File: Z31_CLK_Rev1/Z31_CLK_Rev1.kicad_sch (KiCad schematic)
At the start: 16 parts, among them J1 Conn_01x06_Male, J2 ICSP, U1 MAX6922, U2 4BT-78Z_6L, U3 ATMEGA328-AURCT-ND, U4 MCP2510, U5 TJR1443, Y1 8MHz, Y2 16MHz

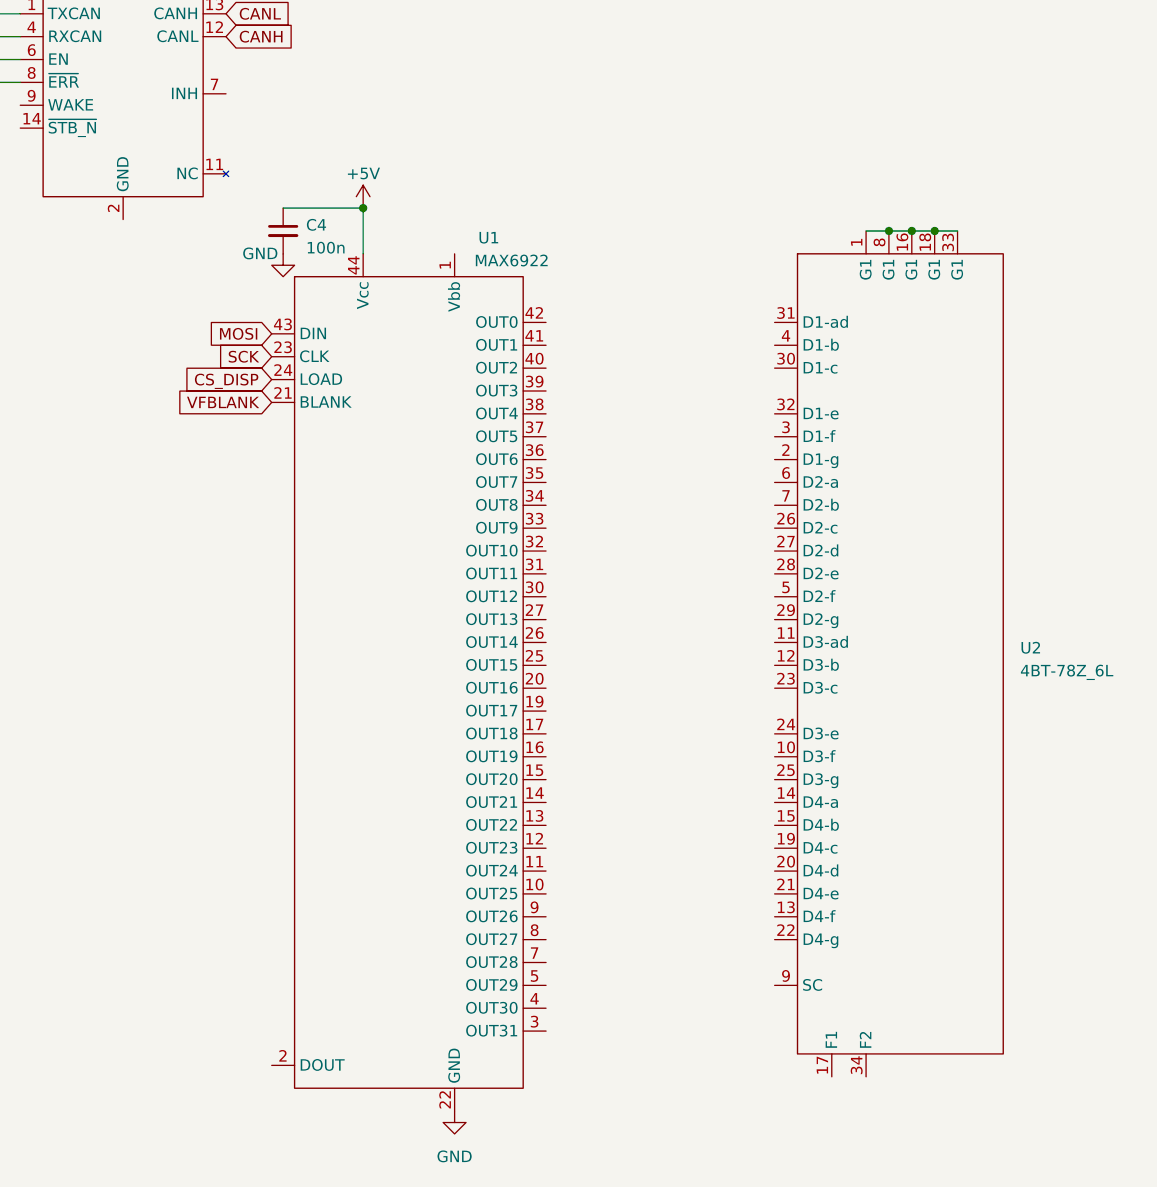
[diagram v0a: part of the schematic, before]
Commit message: add code
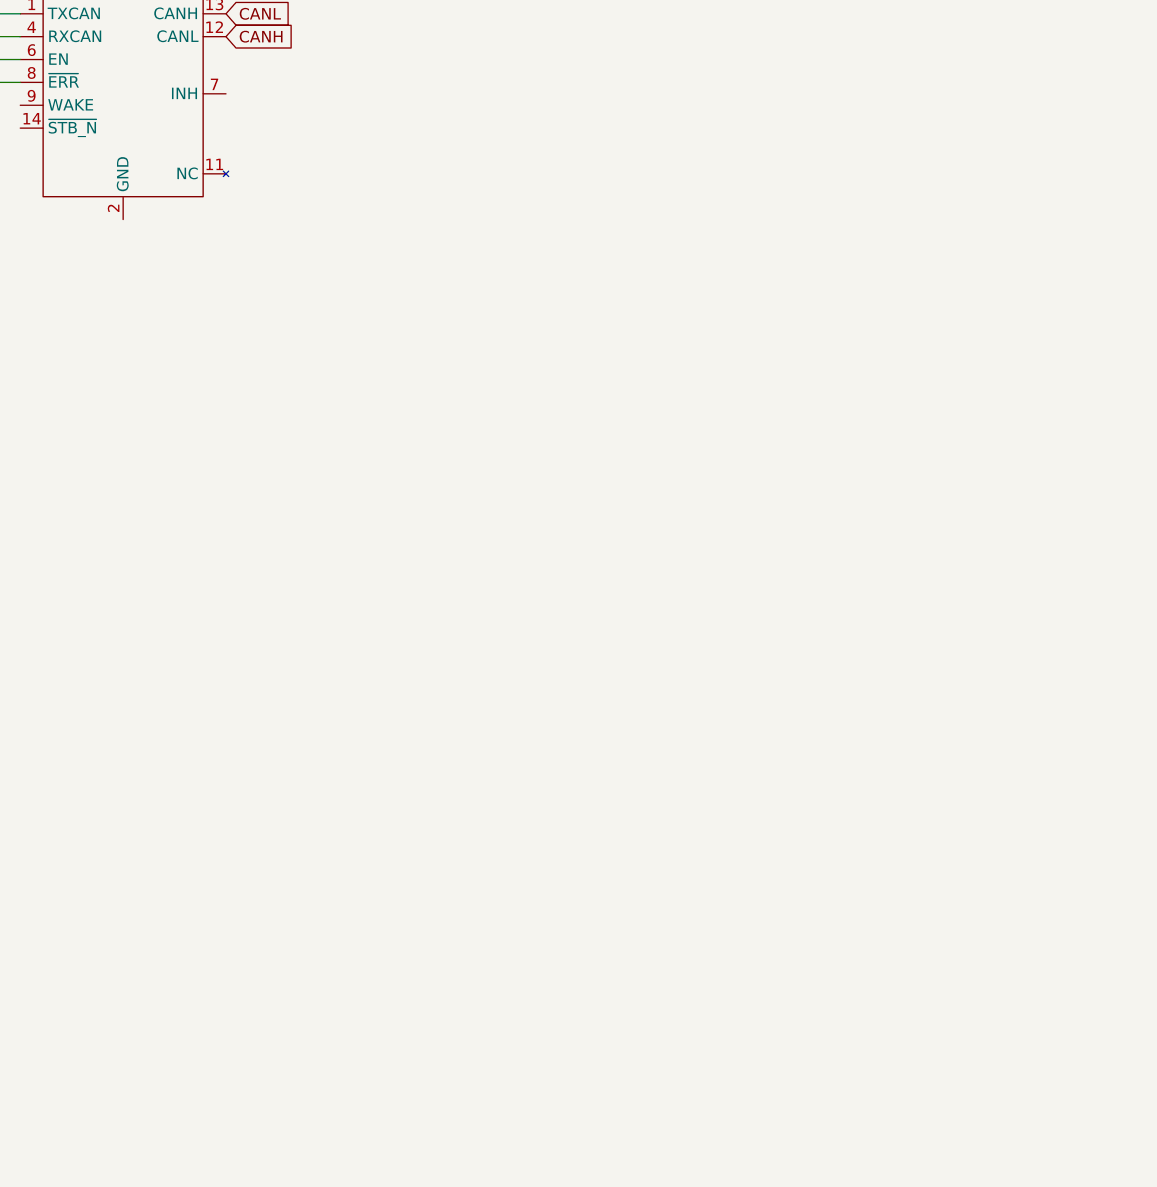
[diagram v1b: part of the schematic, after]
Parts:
- removed C4: 100n, Capacitor_SMD:C_0805_2012Metric_Pad1.18x1.45mm_HandSolder, symbol Device:C_Small
- removed U1: MAX6922, Package_LCC:PLCC-44_16.6x16.6mm_P1.27mm, symbol Personal:MAX6922
- removed U2: 4BT-78Z_6L, Personal:4BT-78Z_6L, symbol Personal:4BT-78Z_6L

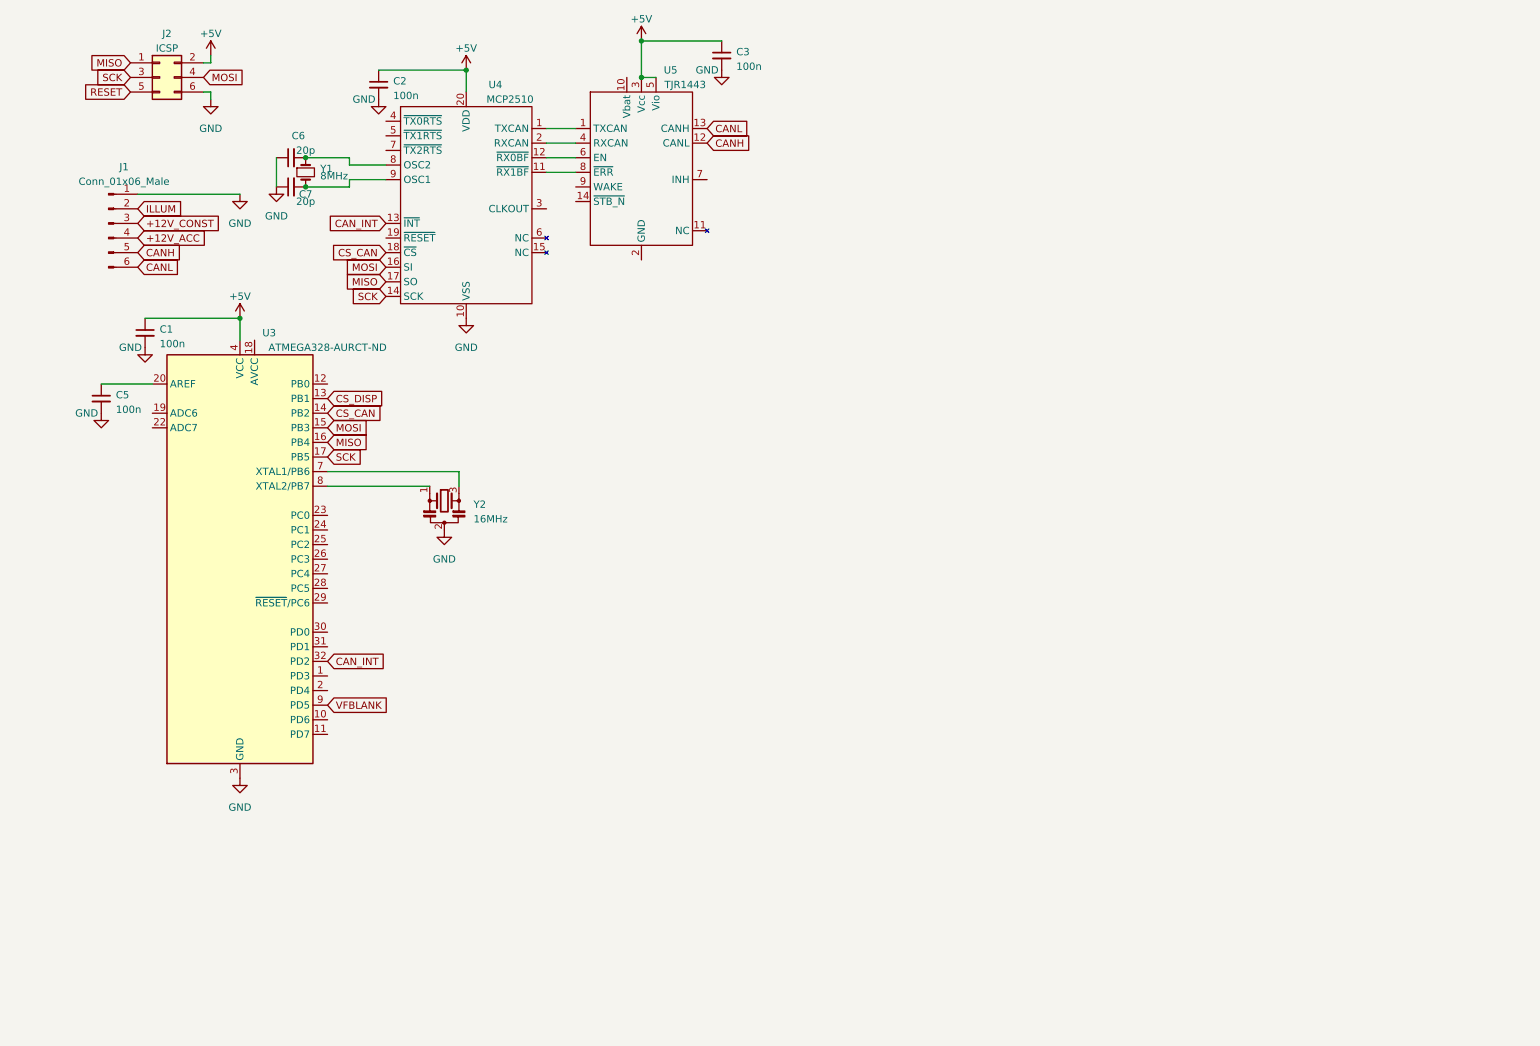
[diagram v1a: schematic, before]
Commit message: Catchup
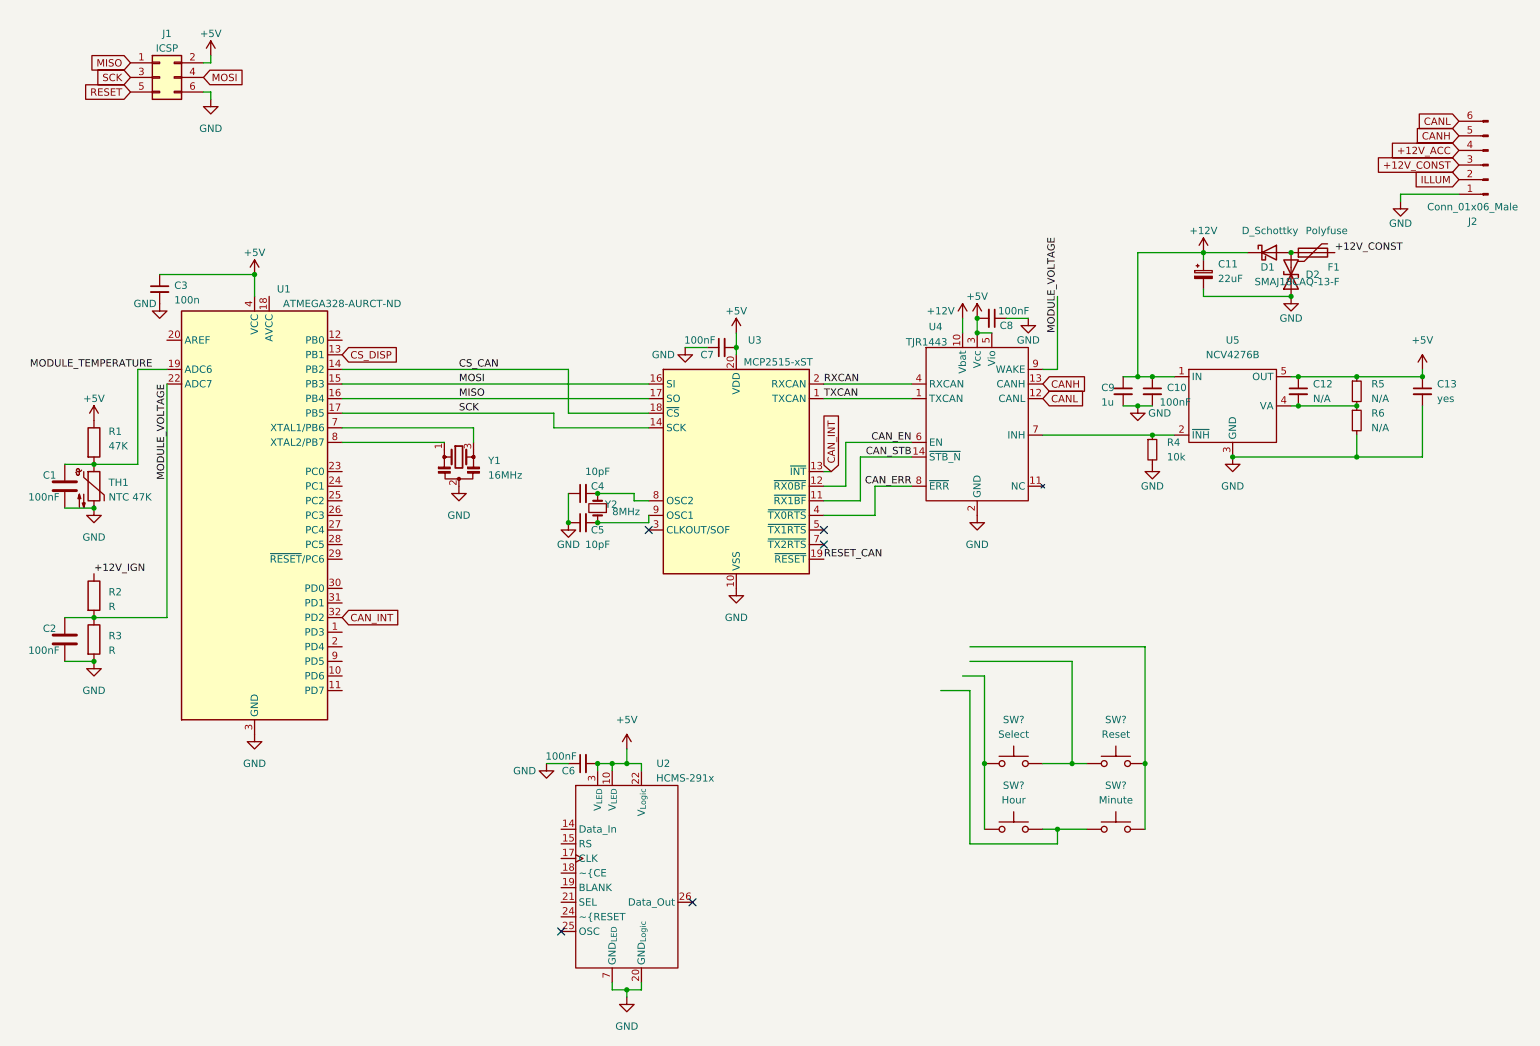
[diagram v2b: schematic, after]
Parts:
- removed C2, C3: 100n, Capacitor_SMD:C_0805_2012Metric_Pad1.18x1.45mm_HandSolder, symbol Device:C_Small
- removed U4: MCP2510, Package_SO:TSSOP-20_4.4x6.5mm_P0.65mm, symbol Personal:MCP2510
- removed U5: TJR1443, Package_SO:SO-14_3.9x8.65mm_P1.27mm, symbol Personal:TJR1443
- removed Y1: 8MHz, Crystal:Crystal_SMD_HC49-SD, symbol Device:Crystal_Small
- added C1, C2: 100nF, Capacitor_SMD:C_0805_2012Metric_Pad1.18x1.45mm_HandSolder, symbol Device:C
- added C10, C8: 100nF, Capacitor_SMD:C_0805_2012Metric_Pad1.18x1.45mm_HandSolder, symbol Device:C_Small
- added C11: 22uF, Capacitor_SMD:CP_Elec_5x5.7, symbol Device:C_Polarized_Small
- added C12: N/A, Capacitor_SMD:C_0805_2012Metric_Pad1.18x1.45mm_HandSolder, symbol Device:C_Small
- added C13: yes, Capacitor_SMD:C_1210_3225Metric_Pad1.33x2.70mm_HandSolder, symbol Device:C_Small
- added C4: 10pF, Capacitor_SMD:C_0805_2012Metric_Pad1.18x1.45mm_HandSolder, symbol Device:C_Small
- added C9: 1u, Capacitor_SMD:C_1210_3225Metric_Pad1.33x2.70mm_HandSolder, symbol Device:C_Small
- added D1: D_Schottky, Diode_SMD:D_SMA, symbol Device:D_Schottky
- added D2: SMAJ18CAQ-13-F, Diode_SMD:D_SMA, symbol Device:D_TVS
- added F1: Polyfuse, Fuse:Fuse_1812_4532Metric_Pad1.30x3.40mm_HandSolder, symbol Device:Polyfuse
- added R1: 47K, Resistor_SMD:R_0805_2012Metric_Pad1.20x1.40mm_HandSolder, symbol Device:R
- added R2, R3: R, Resistor_SMD:R_0805_2012Metric_Pad1.20x1.40mm_HandSolder, symbol Device:R
- added R4: 10k, Resistor_SMD:R_0805_2012Metric_Pad1.20x1.40mm_HandSolder, symbol Device:R_Small
- added R5, R6: N/A, Resistor_SMD:R_0805_2012Metric_Pad1.20x1.40mm_HandSolder, symbol Device:R_Small
- added SW?: Hour, symbol Switch:SW_Push
- added SW?: Select, symbol Switch:SW_Push
- added SW?: Reset, symbol Switch:SW_Push
- added SW?: Minute, symbol Switch:SW_Push
- added TH1: NTC 47K, Resistor_SMD:R_0805_2012Metric_Pad1.20x1.40mm_HandSolder, symbol Device:Thermistor_NTC
- added U2: HCMS-291x, symbol Personal:HCMS-291x
- added U3: MCP2515-xST, Package_SO:TSSOP-20_4.4x6.5mm_P0.65mm, symbol Interface_CAN_LIN:MCP2515-xST
- added U4: TJR1443, Package_SO:SO-14_3.9x8.65mm_P1.27mm, symbol Personal:TJR1443
- added U5: NCV4276B, Package_TO_SOT_SMD:TO-263-5_TabPin3, symbol Personal:NCV4276B
- added Y2: 8MHz, Crystal:Crystal_SMD_HC49-SD, symbol Device:Crystal_Small
- C5: value 100n -> 10pF
- C6, C7: value 20p -> 100nF
- renumbered C1 to C3, J2 to J1, J1 to J2, U3 to U1, Y2 to Y1
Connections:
- net +12V_CONST: now also F1.2
- net +5V: now also C6.2, C7.2, C12.1, C13.1, C8.2, R1.1, R5.1, U2.10 (V_{LED}), U2.22 (V_{Logic}), U2.3 (V_{LED}), U3.20 (VDD), U4.3 (Vcc), U4.5 (Vio), U5.5 (OUT)
- net CANH: now also U4.13 (CANH)
- net CANL: now also U4.12 (CANL)
- net CAN_INT: now also U3.13 (~{INT})
- net CS_CAN: now also U3.18 (~{CS})
- net GND: now also C5.1, C1.2, C10.2, C11.2, C13.2, C2.2, C4.1, C8.1, C9.2, D2.1 (A1), R3.2, R4.2, R6.2, TH1.2, U2.20 (GND_{Logic}), U2.7 (GND_{LED}), U3.10 (VSS), U4.2 (GND), U5.3 (GND); no longer C5.2
- net MISO: now also U3.17 (SO)
- net MOSI: now also U3.16 (SI)
- net SCK: now also U3.14 (SCK)
- net at U1.20 (AREF): no longer C5.1
- net MODULE_TEMPERATURE: now reaches U1.19 (ADC6)
- net MODULE_TEMPERATURE: now also C1.1, R1.2, TH1.1
- net MODULE_VOLTAGE: now reaches U1.22 (ADC7)
- net MODULE_VOLTAGE: now also C2.1, R2.2, R3.1, U4.9 (WAKE)
- net VFBLANK: no longer names the net of U1.9 (PD5)
- new net: R4.1, U4.7 (INH), U5.2 (~{INH})
- new net: C12.2, R5.2, R6.1, U5.4 (VA)
- new net: SW?.1, SW?.1
- new net: SW?.1, SW?.2 (x2)
- new net: SW?.2, SW?.2
- new net: D1.2 (A), D2.2 (A2), F1.1
- new net: C5.2, U3.9 (OSC1), Y2.1
- new net: C4.2, U3.8 (OSC2), Y2.2
- new net +12V: C10.1, C11.1, C9.1, D1.1 (K), U4.10 (Vbat), U5.1 (IN)
- new net +12V_IGN: R2.1
- new net CAN_EN: U3.12 (~{RX0BF}), U4.6 (EN)
- new net CAN_ERR: U3.4 (~{TX0RTS}), U4.8 (~{ERR})
- new net CAN_STB: U3.11 (~{RX1BF}), U4.14 (~{STB_N})
- new net RESET_CAN: U3.19 (~{RESET})
- new net RXCAN: U3.2 (RXCAN), U4.4 (RXCAN)
- new net TXCAN: U3.1 (TXCAN), U4.1 (TXCAN)
- no-connect marks 0 -> 5
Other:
- moved on the sheet: C3, J2, U1, Y1
